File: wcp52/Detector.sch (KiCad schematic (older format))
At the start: 13 parts, among them U10 AD8310ARMZ

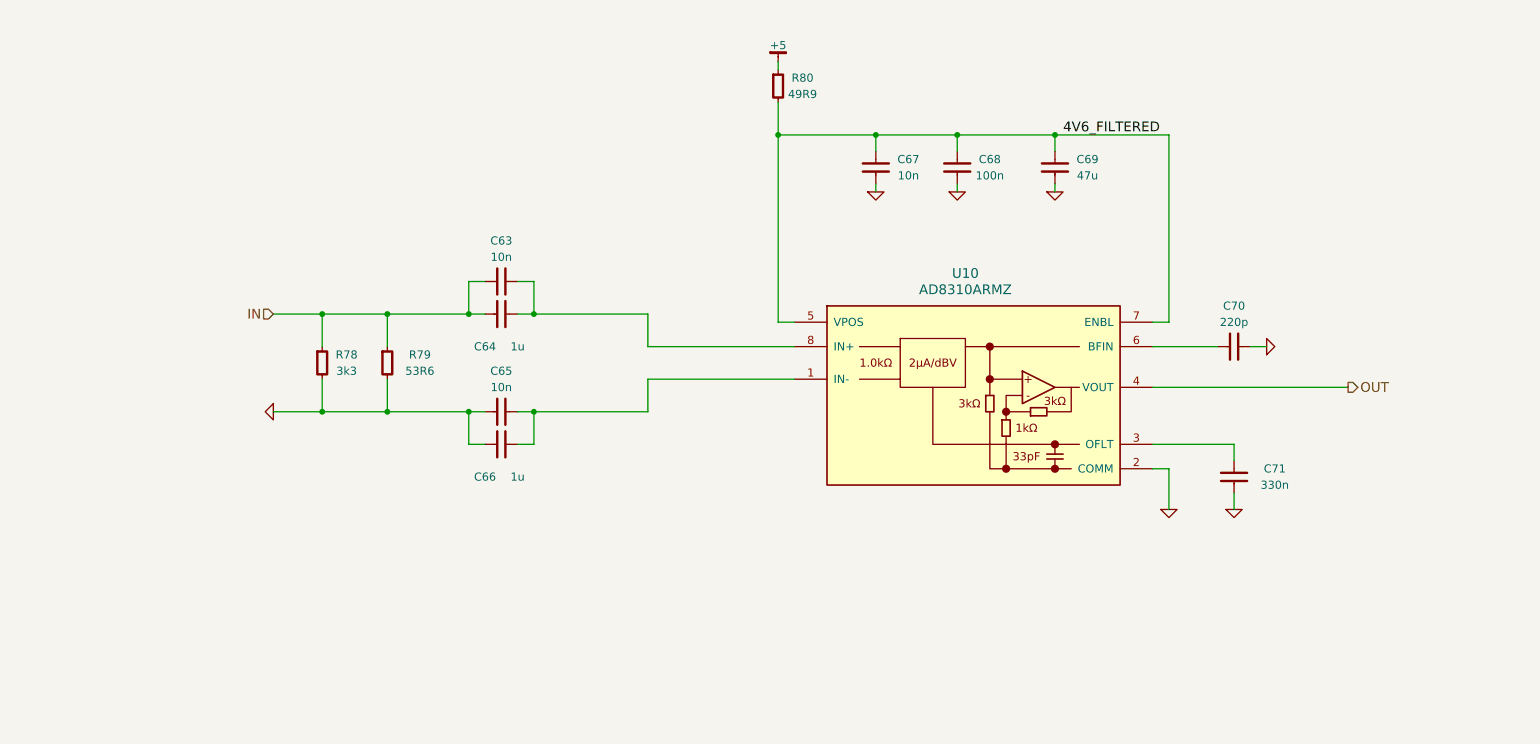
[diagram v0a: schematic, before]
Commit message: Schematic touchups
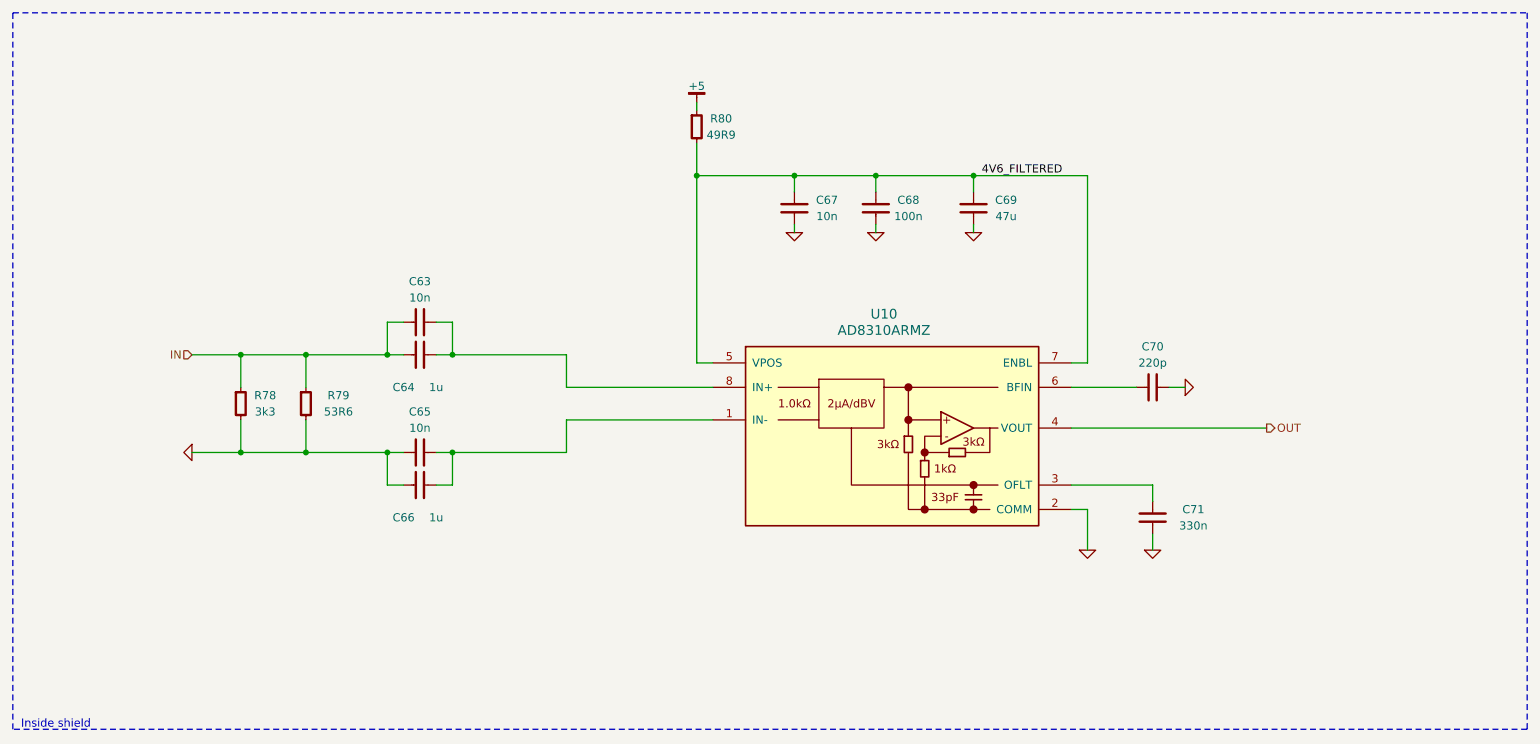
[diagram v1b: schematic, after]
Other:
- note added: "Inside shield"
- moved on the sheet: C63, C64, C65, C66, C67, C68, C69, C70, C71, R78, R79, R80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
